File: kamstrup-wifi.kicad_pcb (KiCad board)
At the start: 2 copper layers, 36 x 89.3 mm, 23 parts, among them T1 BT137, T2 BT137, U1 ESP8266-07

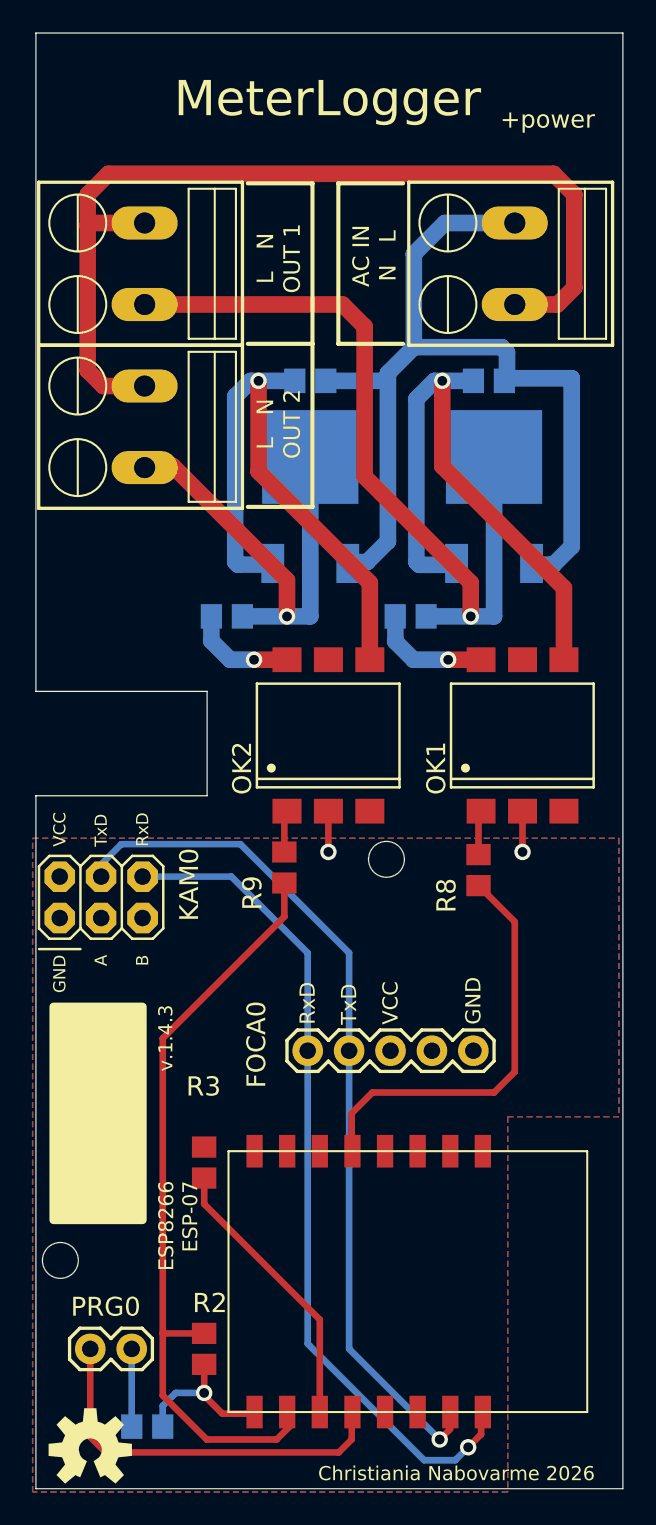
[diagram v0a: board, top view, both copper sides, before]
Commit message: updated pcb+power
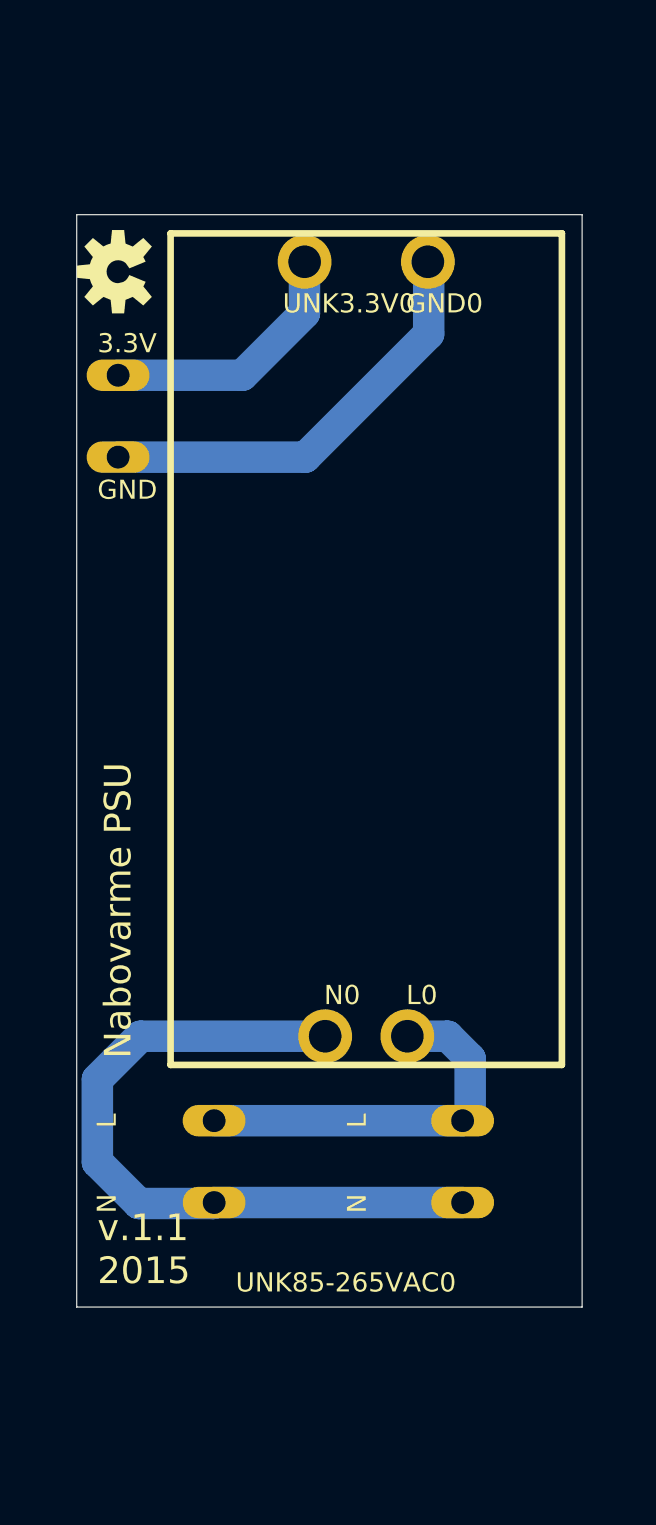
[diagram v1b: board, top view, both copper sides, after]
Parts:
- removed FOCA0: , kamstrup-wifi-import-fps:1X05
- removed JP1: AC IN, kamstrup-wifi-import-fps:SCREWTERMINAL-5MM-2
- removed JP3: AC OUT 2, kamstrup-wifi-import-fps:SCREWTERMINAL-5MM-2
- removed KAM0: , kamstrup-wifi-import-fps:2X03
- removed OK1, OK2: MOC3063S, kamstrup-wifi-import-fps:DIL6-SMD
- removed PRG0: M02PTH, kamstrup-wifi-import-fps:1X02
- removed R1, R2, R3: 10k, kamstrup-wifi-import-fps:R0805
- removed R4, R5, R6, R7: 330, kamstrup-wifi-import-fps:R0805
- removed R8, R9: 120, kamstrup-wifi-import-fps:R0805
- removed T1, T2: BT137, kamstrup-wifi-import-fps:SOT428
- removed U$2: , kamstrup-wifi-import-fps:OSHW-LOGO-M
- removed U1: ESP8266-07, kamstrup-wifi-import-fps:ESP-07
- removed UNK_HOLE_0: , kamstrup-wifi-import-fps:dummyfp0
- removed UNK_HOLE_1: , kamstrup-wifi-import-fps:dummyfp1
- added GND0: M01PTH_2MM, 1X01_2MM, F.Cu at (154.5, 74.4)
- added L0: M01PTH_2MM, 1X01_2MM, F.Cu at (153.3, 121.9)
- added N0: M01PTH_2MM, 1X01_2MM, F.Cu at (148.2, 121.9)
- added U$1: , OSHW-LOGO-M, F.Cu at (135.5, 75.0)
- added UNK3.3V0: M01PTH_2MM, 1X01_2MM, F.Cu at (147.0, 74.4)
- added UNK85-265VAC0: , 1X02_LONGPADS, F.Cu at (156.7, 127.1)
- added UNK85-265VAC1: , 1X02_LONGPADS, F.Cu at (141.4, 127.1)
- JP2: value AC OUT 1 -> (none); footprint kamstrup-wifi-import-fps:SCREWTERMINAL-5MM-2 -> 1X02_LONGPADS
- moved JP2 4.63 mm to (135.5, 81.4), turned to -90 degrees
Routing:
- net N$9: track 56.9 -> 0.00 mm
- net N$16: track 47.3 -> 0.00 mm
- net N$13: track 36.8 -> 0.00 mm, vias 1 -> 0
- net N$6: track 36.5 -> 0.00 mm, vias 1 -> 0
- net N$3: track 48.5 -> 16.2 mm, vias 1 -> 0
- net N$4: track 58.9 -> 26.6 mm
- net N$1: track 51.7 -> 23.7 mm, vias 1 -> 0
- net N$8: track 27.7 -> 0.00 mm, vias 1 -> 0
- net N$11: track 25.7 -> 0.00 mm
- net N$3 (its old number): track 23.8 -> 0.00 mm
- net N$21: track 17.3 -> 0.00 mm
- net GND: track 16.0 -> 0.00 mm, vias 3 -> 0
- net N$2: track 53.3 -> 43.6 mm, vias 1 -> 0
- net N$14: track 7.27 -> 0.00 mm, vias 1 -> 0
- net N$7: track 6.62 -> 0.00 mm, vias 1 -> 0
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- removed copper zone on F.Cu, net 3.3V
- removed copper zone on B.Cu, net GND
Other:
- board size 36 x 89.3 mm -> 31 x 67 mm
- board text added: "3.3V"
- board text added: "L"
- board text added: "N"
- board text added: "Nabovarme PSU"
- board text added: "v.1.1 2015"
- board text removed: "+power"
- board text removed: "A"
- board text removed: "AC IN N L"
- board text removed: "B"
- board text removed: "Christiania Nabovarme 2026"
- board text removed: "ESP8266 ESP-07"
- board text removed: "L N OUT 1"
- board text removed: "L N OUT 2"
- board text removed: "MeterLogger"
- board text removed: "Part RS# JP1, JP2, JP3 821-8701 KAM 702-2937 OK1, OK2 691-2319 R1, R2, R3 721-7820 R4, R5, R6, R7 721-7707 R8, R9 721-6867 T1, T2 792-0709"
- board text removed: "RxD"
- board text removed: "TxD"
- board text removed: "VCC"
- board text removed: "v.1.4.3"
